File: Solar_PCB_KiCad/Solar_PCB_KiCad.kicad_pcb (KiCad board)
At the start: 2 copper layers, 22 parts, among them J1 Screw_Terminal_01x02, J2 Screw_Terminal_01x02, J3 Screw_Terminal_01x02, U1 LT3652EMSE

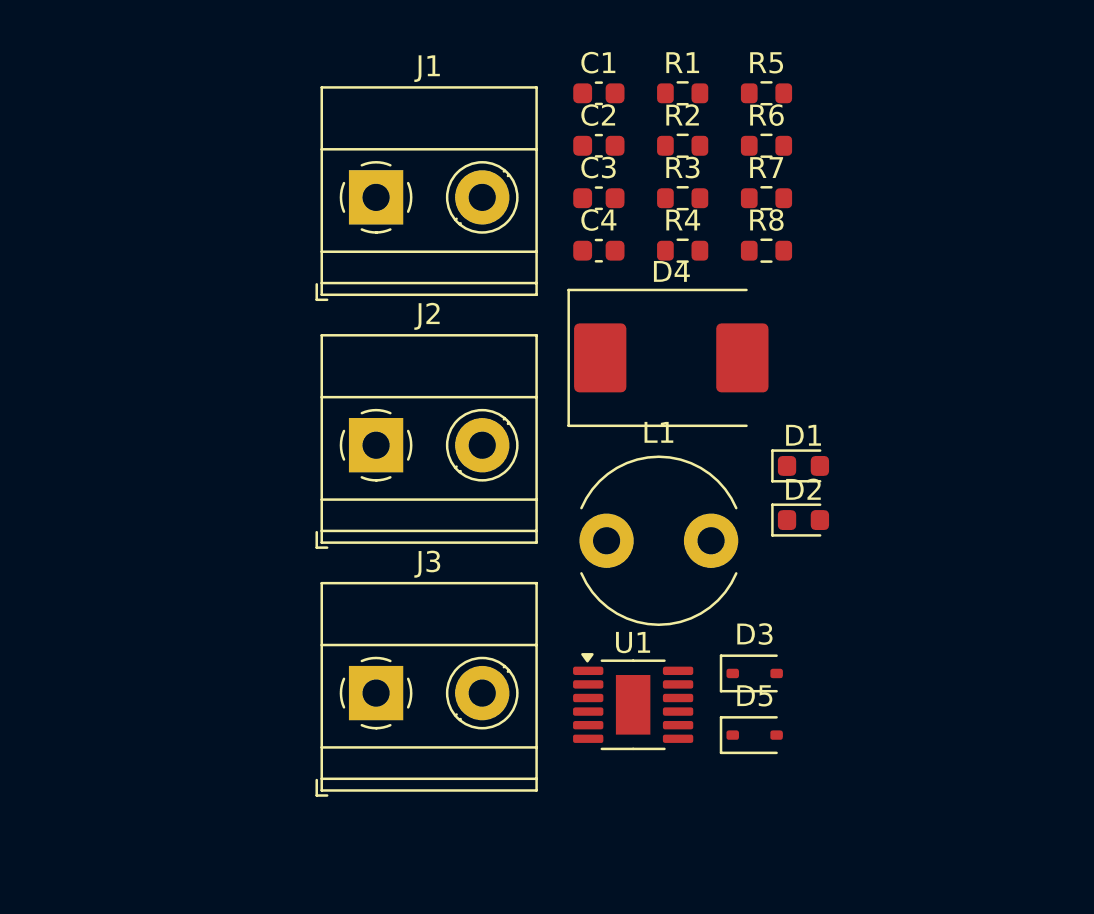
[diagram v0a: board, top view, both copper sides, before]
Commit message: Updated PCB Layout
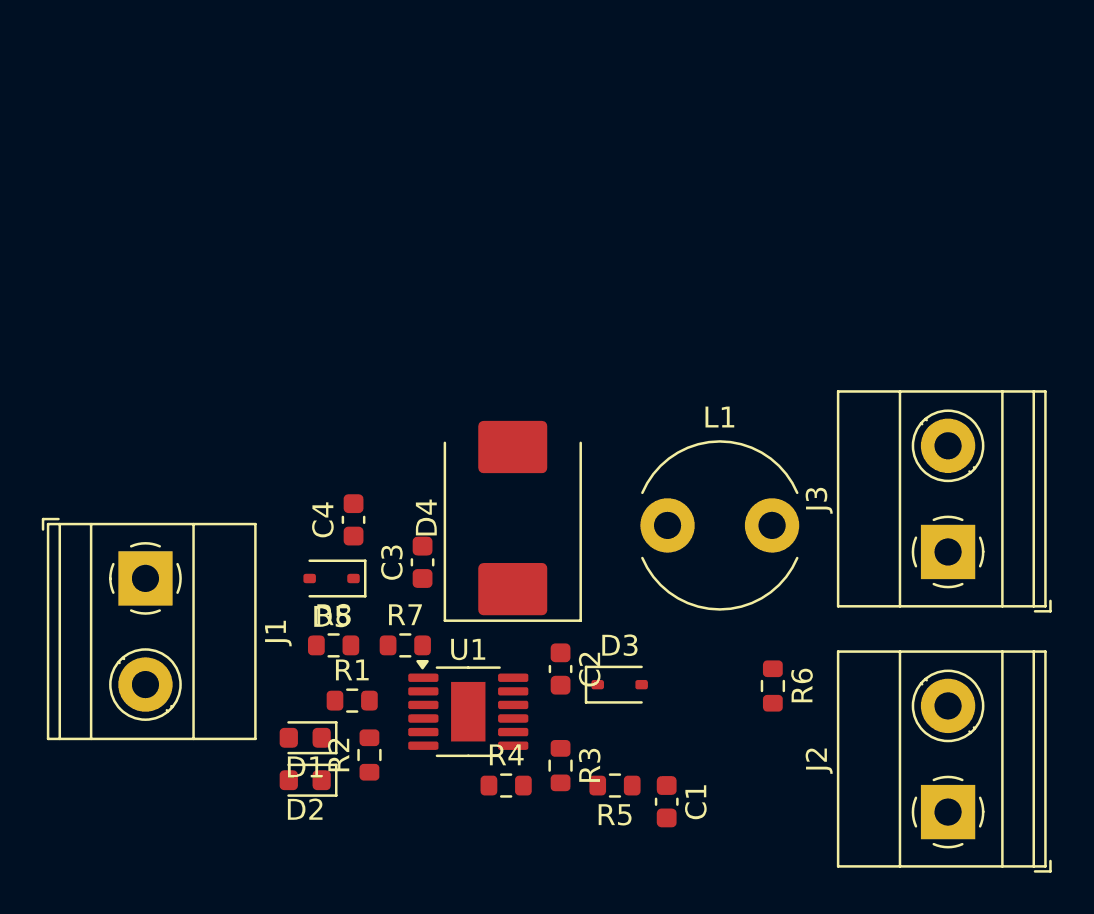
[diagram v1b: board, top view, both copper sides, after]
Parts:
- moved C1 34.1 mm to (157.2, 120.4), turned to -90 degrees
- moved R5 33.9 mm to (154.7, 119.6), turned to 180 degrees
- moved R1 33.1 mm to (142.2, 115.6)
- moved R2 32.8 mm to (143.0, 118.2), turned to 90 degrees
- moved J2 32.5 mm to (170.7, 120.9), turned to 90 degrees
- moved J3 28.2 mm to (170.7, 108.5), turned to 90 degrees
- moved R8 28.0 mm to (141.3, 112.9)
- moved R3 27.8 mm to (152.1, 118.7), turned to -90 degrees
- moved R7 27.5 mm to (144.7, 112.9)
- moved D1 27.2 mm to (139.9, 117.3), turned to 180 degrees
- moved R4 27.0 mm to (149.5, 119.6)
- moved D2 26.9 mm to (139.9, 119.4), turned to 180 degrees
- moved R6 25.9 mm to (162.3, 114.9), turned to -90 degrees
- moved C2 25.1 mm to (152.1, 114.1), turned to -90 degrees
- moved D5 21.6 mm to (141.2, 109.7), turned to 180 degrees
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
